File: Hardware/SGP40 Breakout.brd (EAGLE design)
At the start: 25.4 x 25.4 mm, 48 parts, among them J2 QWIIC_RA, J4 QWIIC_RA, U1 SGP40

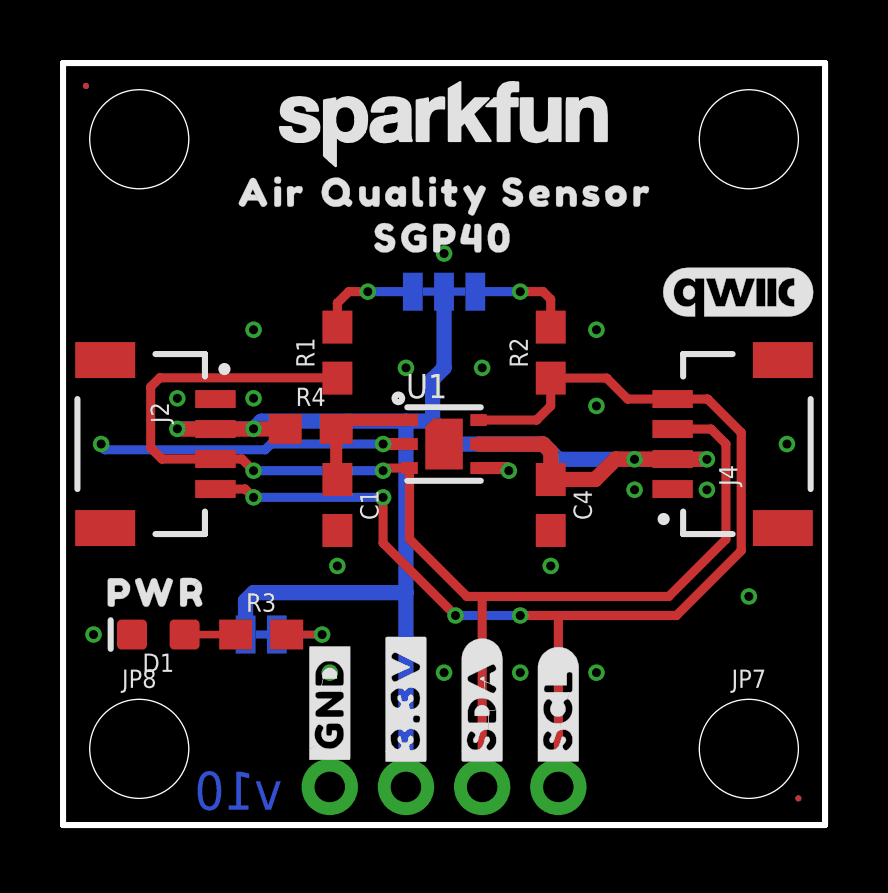
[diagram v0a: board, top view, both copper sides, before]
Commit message: QC Double-check
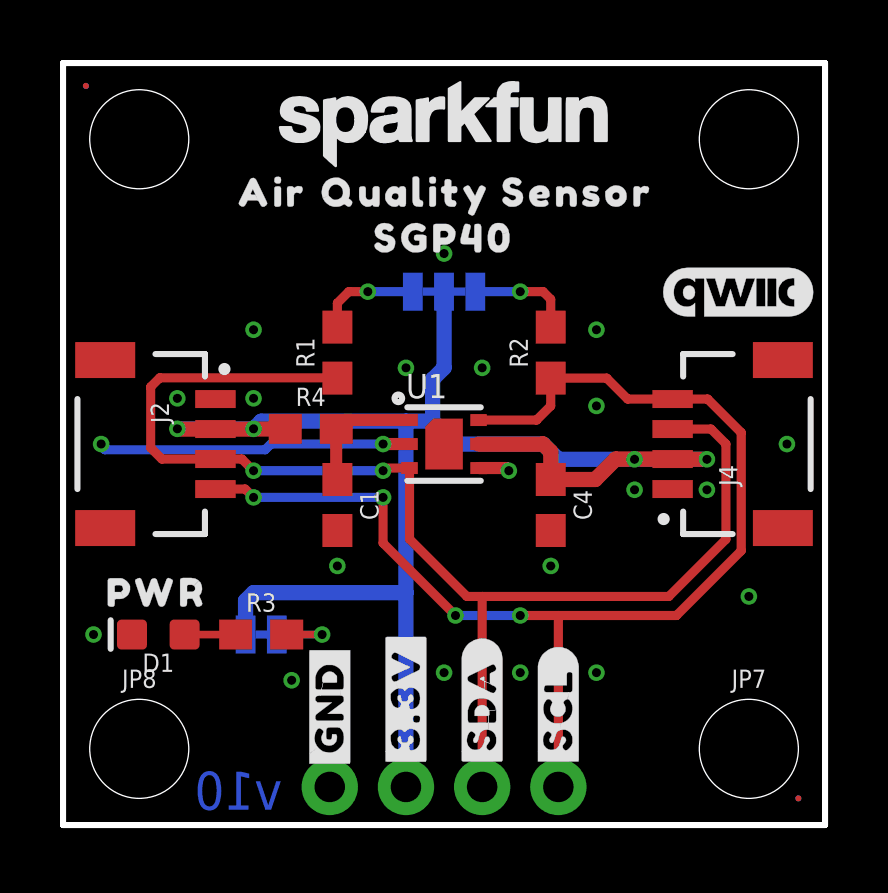
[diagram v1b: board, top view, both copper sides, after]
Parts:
- J1: value (none) -> DNP
- moved U$1 0.13 mm to (8.89, 3.94)
- moved U$33 0.13 mm to (8.89, 3.94)
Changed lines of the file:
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@@
 <drawing>
 <settings>
-<setting alwaysvectorfont="yes"/>
+<setting alwaysvectorfont="no"/>
 <setting keepoldvectorfont="yes"/>
 <setting verticaltext="up"/>
@@
 </element>
 <element name="LOGO5" library="SparkFun-Aesthetics" package="OSHW-LOGO-S" value="OSHW-LOGOS" x="22.86" y="12.7" smashed="yes" rot="MR0"/>
-<element name="J1" library="SparkFun-Connectors" package="1X04_NO_SILK" value="" x="8.89" y="1.27" smashed="yes" rot="MR180">
+<element name="J1" library="SparkFun-Connectors" package="1X04_NO_SILK" value="DNP" x="8.89" y="1.27" smashed="yes" rot="MR180">
 <attribute name="NAME" x="7.62" y="-0.127" size="0.6096" layer="26" font="vector" ratio="20" rot="MR180"/>
 <attribute name="PROD_ID" value="CONN-09696" x="8.89" y="1.27" size="1.778" layer="28" rot="MR180" display="off"/>
@@
 <element name="U$30" library="output" package="SENSOR0" value="" x="21.717" y="15.24" smashed="yes" rot="MR0"/>
 <element name="U$31" library="output" package="ADR#_0X590" value="" x="12.7" y="10.16" smashed="yes" rot="MR0"/>
-<element name="U$33" library="output" package="#GND#0" value="" x="8.89" y="4.064" smashed="yes" rot="R90"/>
+<element name="U$33" library="output" package="#GND#0" value="" x="8.89" y="3.937" smashed="yes" rot="R90"/>
 <element name="U$34" library="output" package="#3#3V#0" value="" x="11.43" y="4.191" smashed="yes" rot="R90"/>
 <element name="U$35" library="output" package="#SDA#0" value="" x="13.97" y="1.778" smashed="yes" rot="R90"/>
 <element name="U$36" library="output" package="#SCL#0" value="" x="16.51" y="1.778" smashed="yes" rot="R90"/>
-<element name="U$1" library="output" package="#GND#0" value="" x="8.89" y="4.064" smashed="yes" rot="MR90"/>
+<element name="U$1" library="output" package="#GND#0" value="" x="8.89" y="3.937" smashed="yes" rot="MR90"/>
 <element name="U$2" library="output" package="#3#3V#0" value="" x="11.43" y="4.191" smashed="yes" rot="MR90"/>
 <element name="U$3" library="output" package="#SDA#0" value="" x="13.97" y="1.778" smashed="yes" rot="MR90"/>
@@
 <via x="15.24" y="5.08" extent="1-16" drill="0.3"/>
 <via x="12.7" y="5.08" extent="1-16" drill="0.3"/>
-<via x="8.89" y="5.08" extent="1-16" drill="0.3"/>
+<via x="7.62" y="4.826" extent="1-16" drill="0.3"/>
 <via x="11.43" y="15.24" extent="1-16" drill="0.3"/>
 <via x="13.97" y="15.24" extent="1-16" drill="0.3"/>
